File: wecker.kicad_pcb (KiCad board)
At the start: 2 copper layers, 85.1 x 31.8 mm, 2 parts, among them J1 Conn_01x20, U1 MSP430FR4133

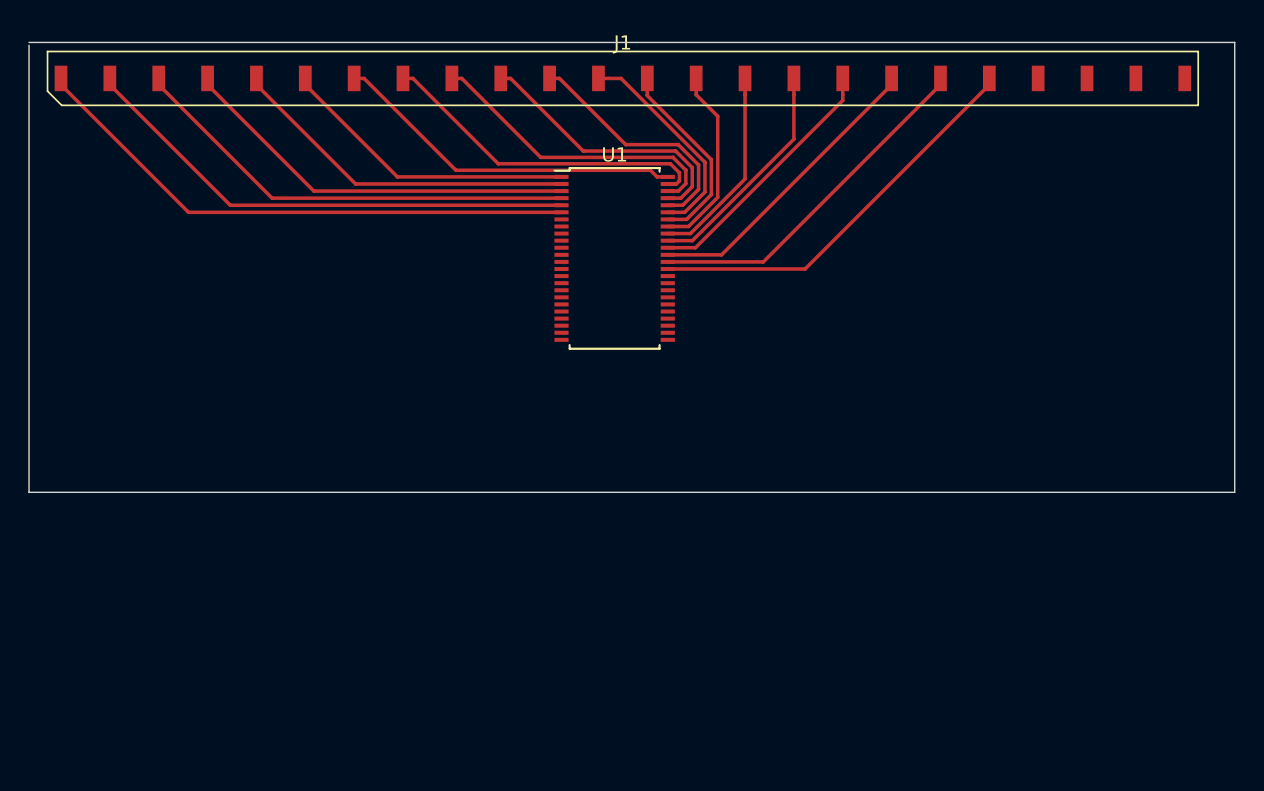
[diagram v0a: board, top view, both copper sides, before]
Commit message: added some more parts
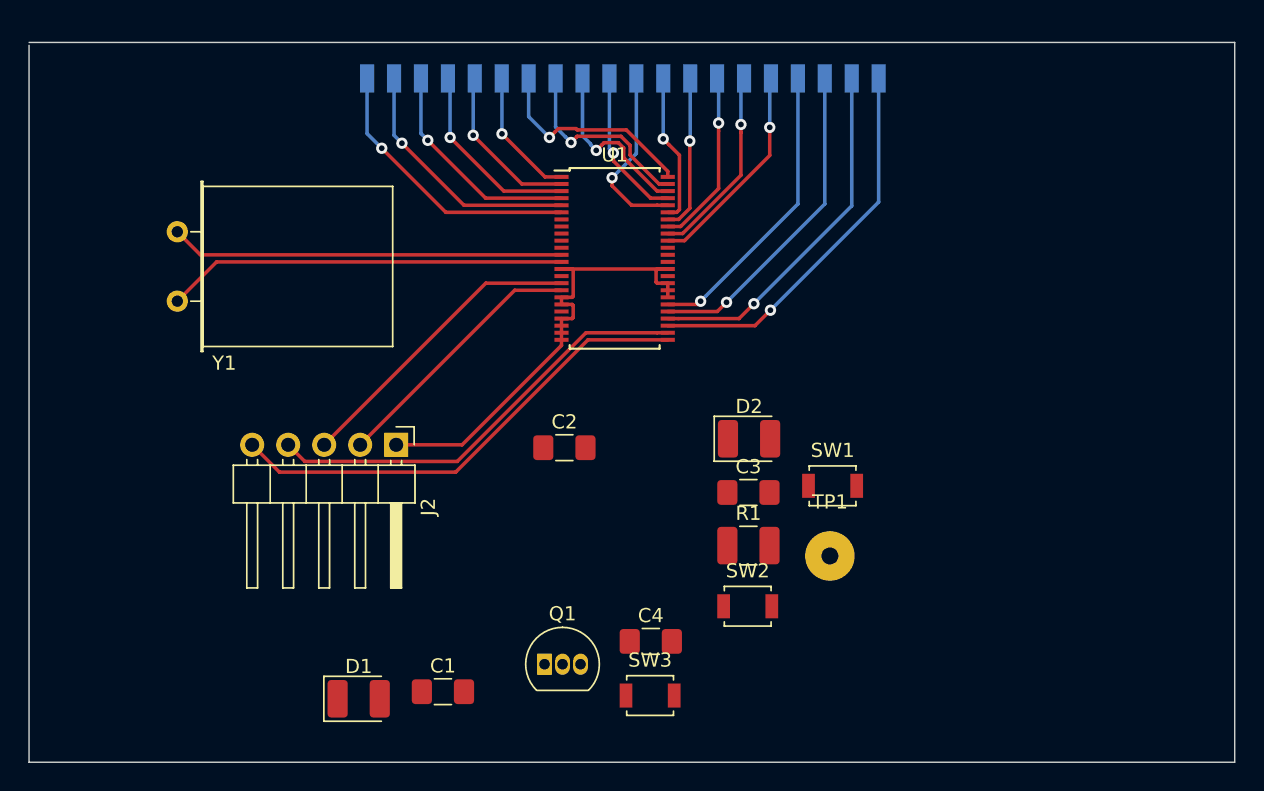
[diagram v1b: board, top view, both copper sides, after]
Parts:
- added C1: 0.1µF, Capacitor_SMD:C_1206_3216Metric_Pad1.42x1.75mm_HandSolder, F.Cu at (96.5, 96.6)
- added C2: 0.1µF, Capacitor_SMD:C_1206_3216Metric_Pad1.42x1.75mm_HandSolder, F.Cu at (105.1, 79.4)
- added C3: 0.1µF, Capacitor_SMD:C_1206_3216Metric_Pad1.42x1.75mm_HandSolder, F.Cu at (118.1, 82.6)
- added C4: 0.1µF, Capacitor_SMD:C_1206_3216Metric_Pad1.42x1.75mm_HandSolder, F.Cu at (111.2, 93.1)
- added D1: LED_BG, LED_SMD:LED_1210_3225Metric_Pad1.42x2.65mm_HandSolder, F.Cu at (90.6, 97.1)
- added D2: LED_BG, LED_SMD:LED_1210_3225Metric_Pad1.42x2.65mm_HandSolder, F.Cu at (118.1, 78.8)
- added J2: Conn_01x05_Male, Connector_PinHeader_2.54mm:PinHeader_1x05_P2.54mm_Horizontal, F.Cu at (93.2, 79.2)
- added Q1: PN2222A, Package_TO_SOT_THT:TO-92_Inline, F.Cu at (103.7, 94.7)
- added R1: R, Resistor_SMD:R_1210_3225Metric_Pad1.42x2.65mm_HandSolder, F.Cu at (118.1, 86.3)
- added SW1: Hour, Button_Switch_SMD:SW_SPST_B3U-1000P, F.Cu at (124.0, 82.1)
- added SW2: Minute, Button_Switch_SMD:SW_SPST_B3U-1000P, F.Cu at (118.0, 90.6)
- added SW3: Snooze, Button_Switch_SMD:SW_SPST_B3U-1000P, F.Cu at (111.1, 96.9)
- added TP1: ClockInput, Connector_Wire:SolderWirePad_1x01_Drill1.2mm, F.Cu at (123.8, 87.0)
- added Y1: 32.768 kHz, Crystal:Crystal_HC18-U_Horizontal, F.Cu at (77.8, 69.1)
- J1: moved to B.Cu
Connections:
- U1 pad 10: (no net) -> Net-(C1-Pad2)
- U1 pad 11: (no net) -> Net-(C1-Pad1)
- U1 pad 12: (no net) -> Net-(U1-Pad12)
- U1 pad 13: (no net) -> Net-(U1-Pad13)
- U1 pad 14: (no net) -> GND
- U1 pad 15: (no net) -> +BATT
- U1 pad 16: (no net) -> Net-(J2-Pad3)
- U1 pad 17: (no net) -> Net-(J2-Pad2)
- U1 pad 18: (no net) -> GND
- U1 pad 19: (no net) -> GND
- U1 pad 20: (no net) -> Net-(TP1-Pad1)
- U1 pad 21: (no net) -> GND
- U1 pad 22: (no net) -> GND
- U1 pad 23: (no net) -> GND
- U1 pad 24: (no net) -> GND
- U1 pad 25: (no net) -> Net-(J2-Pad5)
- U1 pad 26: (no net) -> Net-(J2-Pad4)
- U1 pad 27: (no net) -> Net-(J1-Pad20)
- U1 pad 28: (no net) -> Net-(J1-Pad19)
- U1 pad 29: (no net) -> Net-(J1-Pad18)
- U1 pad 30: (no net) -> Net-(J1-Pad17)
- U1 pad 31: (no net) -> GND
- U1 pad 32: (no net) -> GND
- U1 pad 33: (no net) -> GND
- U1 pad 34: (no net) -> Net-(Q1-Pad2)
- U1 pad 35: Net-(J1-Pad20) -> GND
- U1 pad 36: Net-(J1-Pad19) -> Net-(SW3-Pad1)
- U1 pad 37: Net-(J1-Pad18) -> Net-(SW2-Pad1)
- U1 pad 38: Net-(J1-Pad17) -> Net-(SW1-Pad1)
- U1 pad 7: (no net) -> Net-(C4-Pad1)
- U1 pad 8: (no net) -> Net-(C3-Pad1)
- U1 pad 9: (no net) -> Net-(C2-Pad2)
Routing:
- net GND: track 0.00 -> 34.2 mm
- net Net-(J2-Pad5): track 0.00 -> 34.0 mm
- net Net-(J2-Pad4): track 0.00 -> 31.0 mm
- net Net-(U1-Pad13): track 0.00 -> 28.3 mm
- net Net-(U1-Pad12): track 0.00 -> 27.8 mm
- net Net-(J2-Pad3): track 0.00 -> 21.5 mm
- net Net-(J1-Pad1): track 39.5 -> 19.9 mm, vias 0 -> 1
- net Net-(J2-Pad2): track 0.00 -> 18.7 mm
- net Net-(J1-Pad2): track 35.8 -> 17.9 mm, vias 0 -> 1
- net Net-(J1-Pad3): track 32.2 -> 15.7 mm, vias 0 -> 1
- net Net-(J1-Pad4): track 28.5 -> 13.7 mm, vias 0 -> 1
- net Net-(J1-Pad5): track 24.9 -> 11.7 mm, vias 0 -> 1
- net Net-(J1-Pad6): track 21.2 -> 9.38 mm, vias 0 -> 1
- net Net-(J1-Pad7): track 25.0 -> 15.0 mm, vias 0 -> 1
- net Net-(J1-Pad8): track 23.8 -> 13.8 mm, vias 0 -> 1
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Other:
- board size 85.1 x 31.8 mm -> 85.1 x 50.8 mm
